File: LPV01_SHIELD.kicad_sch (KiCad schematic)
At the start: 123 parts, among them J1 Screw_Terminal_01x02, J10 SPI_header, J11 Power_socket, J15 Inputs, J16 Screw_Terminal_01x02, J17 Wiegand, J2 Screw_Terminal_01x02, J22 Inputs, J23 Screw_Terminal_01x02, J24 Conn_01x02_Pin, J3 Screw_Terminal_01x02, J9 GPIO_header, Q1 BC817, Q10 BC817, Q11 BC817, Q12 BC817, Q13 BC817, Q14 BC817, Q15 BC817, Q2 BC817, Q3 BC817, Q4 TLP521-4XSM, Q5 TLP521-4XSM, Q6 TLP521-4XSM, Q7 BC817, Q8 TLP521-4XSM, Q9 BC817, SW1 SW_SPST, SW10 SW_SPST, SW11 SW_SPST, SW2 SW_SPST, SW3 SW_SPST, SW4 SW_SPST, SW5 SW_SPST, SW6 SW_SPST, SW7 SW_SPST, SW8 SW_SPST, SW9 SW_SPST, U1 TLP175A, U2 TLP175A, U3 TLP175A

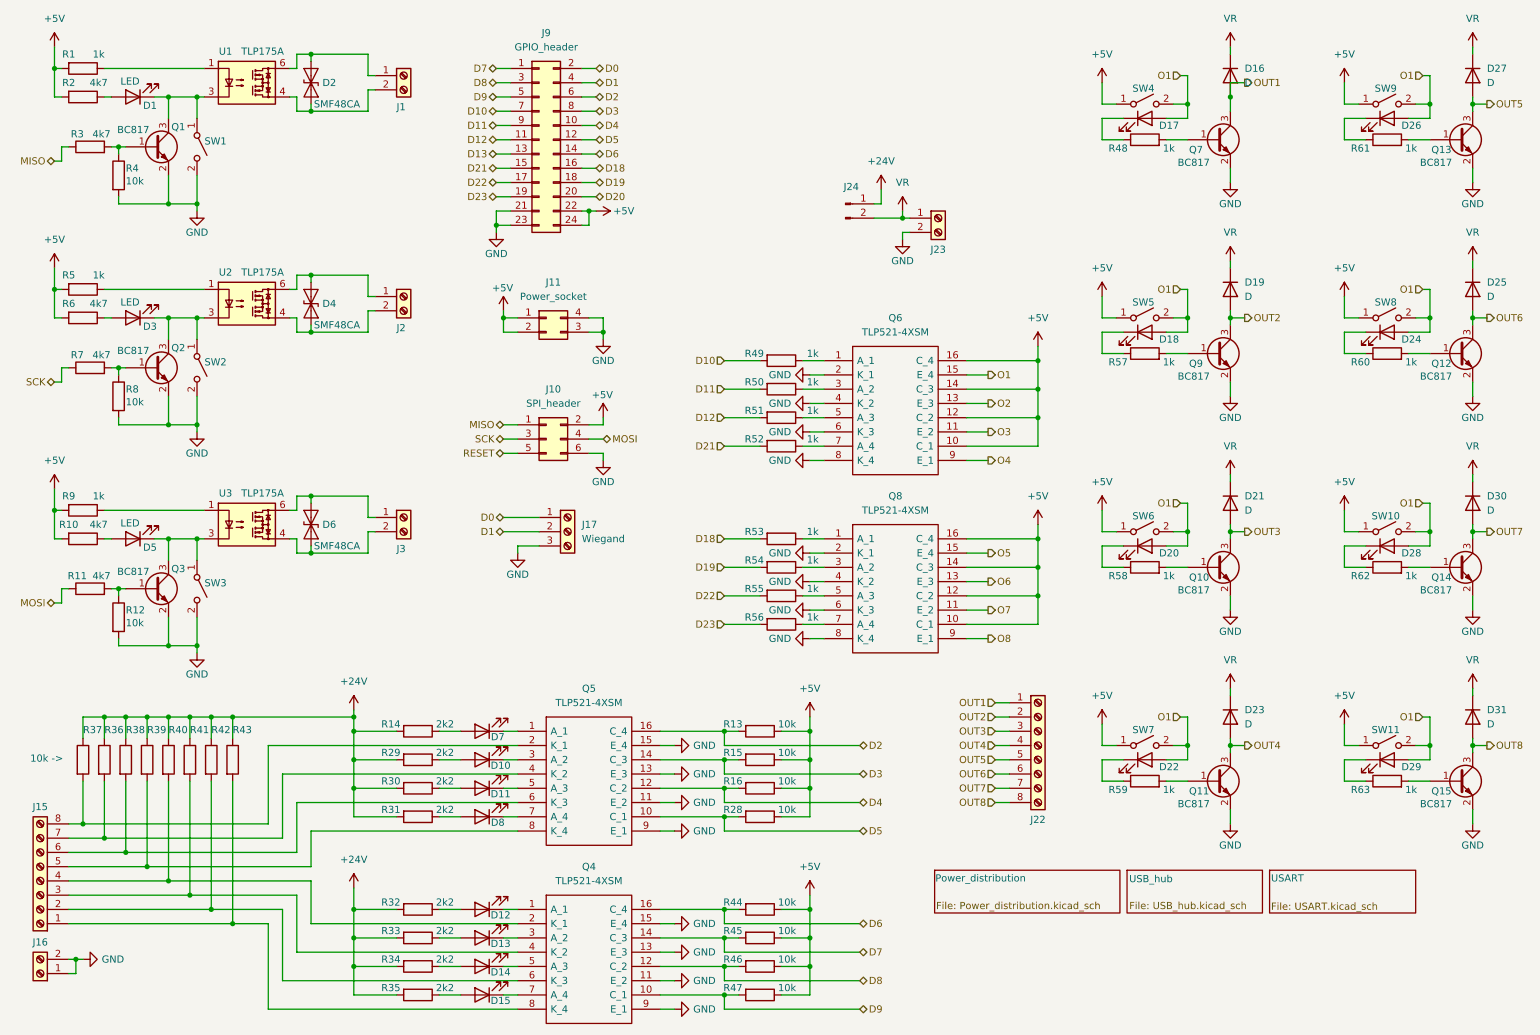
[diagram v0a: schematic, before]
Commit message: PCB rebuilt
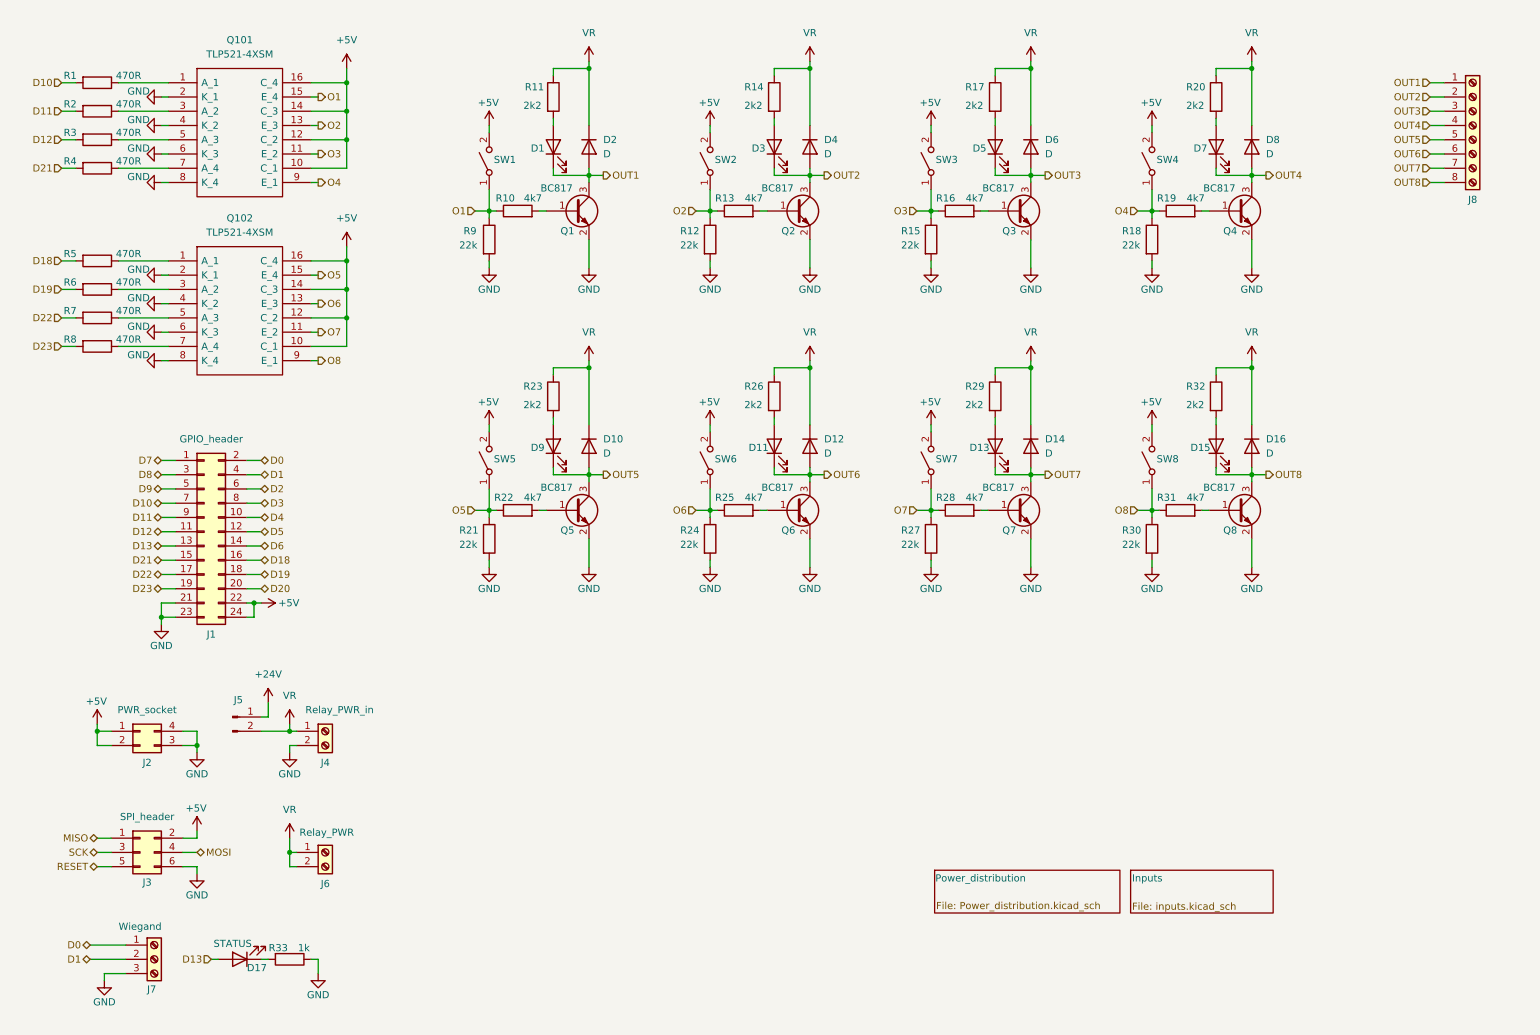
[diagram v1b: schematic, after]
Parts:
- removed D10, D12, D14, D8: LED, symbol Device:LED
- removed D18, D20, D22, D24, D26, D28, D29: LED, LED_SMD:LED_0603_1608Metric, symbol Device:LED
- removed D2, D4, D6: SMF48CA, Diode_SMD:D_SMA, symbol Diode:SD36_SOD323
- removed D21, D23, D25, D27, D30, D31: D, symbol Device:D
- removed J1, J2, J3: Screw_Terminal_01x02, TerminalBlock_Phoenix:TerminalBlock_Phoenix_MKDS-1,5-2_1x02_P5.00mm_Horizontal, symbol Connector:Screw_Terminal_01x02
- removed J15: Inputs, TerminalBlock_Phoenix:TerminalBlock_Phoenix_PT-1,5-8-3.5-H_1x08_P3.50mm_Horizontal, symbol Connector:Screw_Terminal_01x08
- removed J16: Screw_Terminal_01x02, TerminalBlock_Phoenix:TerminalBlock_Phoenix_PT-1,5-2-3.5-H_1x02_P3.50mm_Horizontal, symbol Connector:Screw_Terminal_01x02
- removed Q1, Q10, Q11, Q12, Q13, Q14, Q15: BC817, Package_TO_SOT_SMD:SOT-23, symbol Transistor_BJT:BC817
- removed Q4, Q5, Q6, Q8: TLP521-4XSM, SamacSys_Parts:TLP5214XSM, symbol SamacSys_Parts:TLP521-4XSM
- removed R10: 4k7, Resistor_SMD:R_0603_1608Metric, symbol Device:R
- removed R34, R35: 2k2, Resistor_SMD:R_0603_1608Metric, symbol Device:R
- removed R36, R38, R39, R40, R41, R42, R43, R44, R45, R46, R47: 10k, Resistor_SMD:R_0603_1608Metric, symbol Device:R
- removed R37: 10k ->, Resistor_SMD:R_0603_1608Metric, symbol Device:R
- removed R48, R49, R50, R51, R52, R53, R54, R55, R56, R58, R59, R60, R61, R62, R63: 1k, Resistor_SMD:R_0603_1608Metric, symbol Device:R
- removed SW10, SW11, SW9: SW_SPST, Button_Switch_SMD:SW_SPST_CK_RS282G05A3, symbol Switch:SW_SPST
- removed U1, U2, U3: TLP175A, Package_SO:MFSOP6-4_4.4x3.6mm_P1.27mm, symbol Relay_SolidState:TLP175A
- added D10, D12, D14, D4, D6, D8: D, Diode_SMD:D_MicroMELF, symbol Device:D
- added D9: LED, LED_SMD:LED_0603_1608Metric, symbol Device:LED
- added J6: Relay_PWR, TerminalBlock_Phoenix:TerminalBlock_Phoenix_PT-1,5-2-3.5-H_1x02_P3.50mm_Horizontal, symbol Connector:Screw_Terminal_01x02
- added Q101, Q102: TLP521-4XSM, SamacSys_Parts:TLP5214XSM, symbol SamacSys_Parts:TLP521-4XSM
- added Q4, Q5, Q6, Q8: BC817, Package_TO_SOT_SMD:SOT-23, symbol Transistor_BJT:BC817
- added R17, R20, R23, R26: 2k2, Resistor_SMD:R_0603_1608Metric, symbol Device:R
- added R18, R21, R24, R27: 22k, Resistor_SMD:R_0603_1608Metric, symbol Device:R
- added R19, R22, R25: 4k7, Resistor_SMD:R_0603_1608Metric, symbol Device:R
- D11, D13, D15, D7: footprint (none) -> LED_SMD:LED_0603_1608Metric
- D16: footprint (none) -> Diode_SMD:D_MicroMELF
- D17: value LED -> STATUS
- D2: renamed from D19; footprint (none) -> Diode_SMD:D_MicroMELF
- J2: renamed from J11; value Power_socket -> PWR_socket
- J4: renamed from J23; value Screw_Terminal_01x02 -> Relay_PWR_in
- J5: renamed from J24; footprint (none) -> Connector_PinHeader_2.54mm:PinHeader_1x02_P2.54mm_Vertical
- R1, R5: value 1k -> 470R
- R10: renamed from R57; value 1k -> 4k7
- R11: value 4k7 -> 2k2
- R12, R15: value 10k -> 22k
- R13, R16, R28: value 10k -> 4k7
- R2, R3, R6, R7: value 4k7 -> 470R
- R30: value 2k2 -> 22k
- R31: value 2k2 -> 4k7
- R33: value 2k2 -> 1k
- R4, R8: value 10k -> 470R
- R9: value 1k -> 22k
- renumbered J9 to J1, J10 to J3, J17 to J7, J22 to J8, Q9 to Q1
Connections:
- net +24V: no longer R14.2, R29.2, R30.2, R31.2, R32.2, R33.2
- net +5V: now also SW1.2 (B), SW2.2 (B), SW3.2 (B), SW4.2 (B), SW5.2 (B), SW6.2 (B), SW7.2 (B), SW8.2 (B), Q101.10 (C_1), Q101.12 (C_2), Q101.14 (C_3), Q101.16 (C_4), Q102.10 (C_1), Q102.12 (C_2), Q102.14 (C_3), Q102.16 (C_4); no longer R1.2, R13.1, R15.1, R16.1, R2.2, R28.1, R5.2, R6.2, R9.2, SW4.1 (A), SW5.1 (A), SW6.1 (A), SW7.1 (A), SW8.1 (A)
- net D10: now also R1.2
- net D11: now also R2.2
- net D12: now also R3.2
- net D13: now also D17.2 (A)
- net D18: now also R5.2
- net D19: now also R6.2
- net D2: no longer R13.2
- net D21: now also R4.2
- net D22: now also R7.2
- net D23: now also R8.2
- net D3: no longer R15.2
- net D4: no longer R16.2
- net D5: no longer R28.2
- net GND: now also R15.2, R30.2, R33.1, R9.2, Q101.2 (K_1), Q101.4 (K_2), Q101.6 (K_3), Q101.8 (K_4), Q102.2 (K_1), Q102.4 (K_2), Q102.6 (K_3), Q102.8 (K_4), Q4.2 (E), Q5.2 (E), Q6.2 (E), Q8.2 (E), R18.2, R21.2, R24.2, R27.2; no longer R4.2, R8.2, SW1.2 (B), SW2.2 (B), SW3.2 (B)
- net MISO: no longer R3.1
- net MOSI: no longer R11.1
- net O1: now also R10.1, R9.1, SW1.1 (A), Q101.15 (E_4); no longer D17.2 (A), SW4.2 (B), SW5.2 (B), SW6.2 (B), SW7.2 (B), SW8.2 (B)
- net O2: now also R12.1, R13.1, SW2.1 (A), Q101.13 (E_3)
- net O3: now also R15.1, R16.1, SW3.1 (A), Q101.11 (E_2)
- net O4: now also SW4.1 (A), Q101.9 (E_1), R18.1, R19.1
- net O5: now also SW5.1 (A), Q102.15 (E_4), R21.1, R22.1
- net O6: now also SW6.1 (A), Q102.13 (E_3), R24.1, R25.1
- net O7: now also R28.1, SW7.1 (A), Q102.11 (E_2), R27.1
- net O8: now also R30.1, R31.1, SW8.1 (A), Q102.9 (E_1)
- net OUT1: now also D1.1 (K), D2.2 (A), Q1.3 (C); no longer D16.2 (A), Q7.3 (C)
- net OUT2: now also D3.1 (K), Q2.3 (C), D4.2 (A); no longer D2.2 (A), Q1.3 (C)
- net OUT3: now also D5.1 (K), Q3.3 (C), D6.2 (A)
- net OUT4: now also D7.1 (K), D8.2 (A), Q4.3 (C)
- net OUT5: now also D10.2 (A), D9.1 (K), Q5.3 (C)
- net OUT6: now also D11.1 (K), D12.2 (A), Q6.3 (C)
- net OUT7: now also D13.1 (K), Q7.3 (C), D14.2 (A)
- net OUT8: now also D15.1 (K), D16.2 (A), Q8.3 (C)
- net SCK: no longer R7.1
- net VR: now also R11.1, R14.1, R29.1, R32.1, D10.1 (K), D12.1 (K), D14.1 (K), D4.1 (K), D6.1 (K), D8.1 (K), J6.1 (Pin_1), J6.2 (Pin_2), R17.1, R20.1, R23.1, R26.1
- net at R4.1: now also Q101.7 (A_4); no longer R3.2
- net at Q7.1 (B): now also R28.2
- net at D15.2 (A): now also R32.2
- net at D17.1 (K): now also R33.2
- net at D11.2 (A): now also R26.2; no longer R30.1
- net at D5.2 (A): now also R17.2
- net at R6.1: now also Q102.3 (A_2); no longer D3.2 (A)
- net at R5.1: now also Q102.1 (A_1)
- net at R1.1: now also Q101.1 (A_1)
- net at D13.2 (A): now also R29.2; no longer R33.1
- net at D7.2 (A): now also R20.2; no longer R14.1
- net at R2.1: now also Q101.3 (A_2); no longer D1.2 (A)
- new net: Q6.1 (B), R25.2
- new net: Q8.1 (B), R31.2
- new net: D9.2 (A), R23.2
- new net: Q4.1 (B), R19.2
- new net: Q5.1 (B), R22.2
- new net: Q102.7 (A_4), R8.1
- new net: Q3.1 (B), R16.2
- new net: D1.2 (A), R11.2
- new net: Q101.5 (A_3), R3.1
- new net: Q102.5 (A_3), R7.1
- new net: D3.2 (A), R14.2
- new net: Q2.1 (B), R13.2
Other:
- removed sheet USART
- removed sheet USB_hub
- added sheet Inputs (inputs.kicad_sch)
- moved on the sheet: D2, J1, J2, J3, J4, J5, J7, J8, Q1, R10
